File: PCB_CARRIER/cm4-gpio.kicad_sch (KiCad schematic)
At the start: 35 parts, among them J2 Micro_SD_Card_Det2, Q1 BSS138, Q2 BSS138, Q3 BSS138, Q4 BC817-40, SW1 SW_DIP_x04, U4 RT9742GGJ5

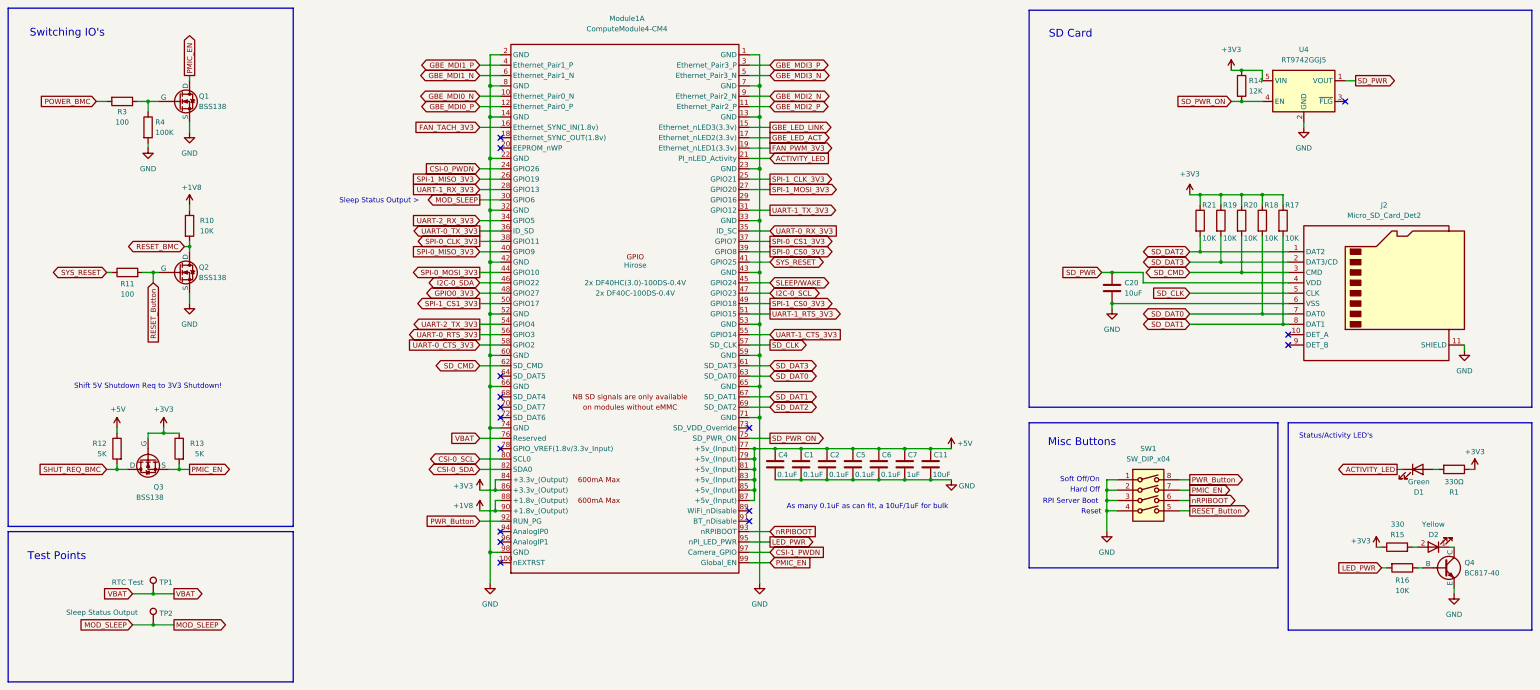
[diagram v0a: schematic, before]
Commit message: fixing another mosfet
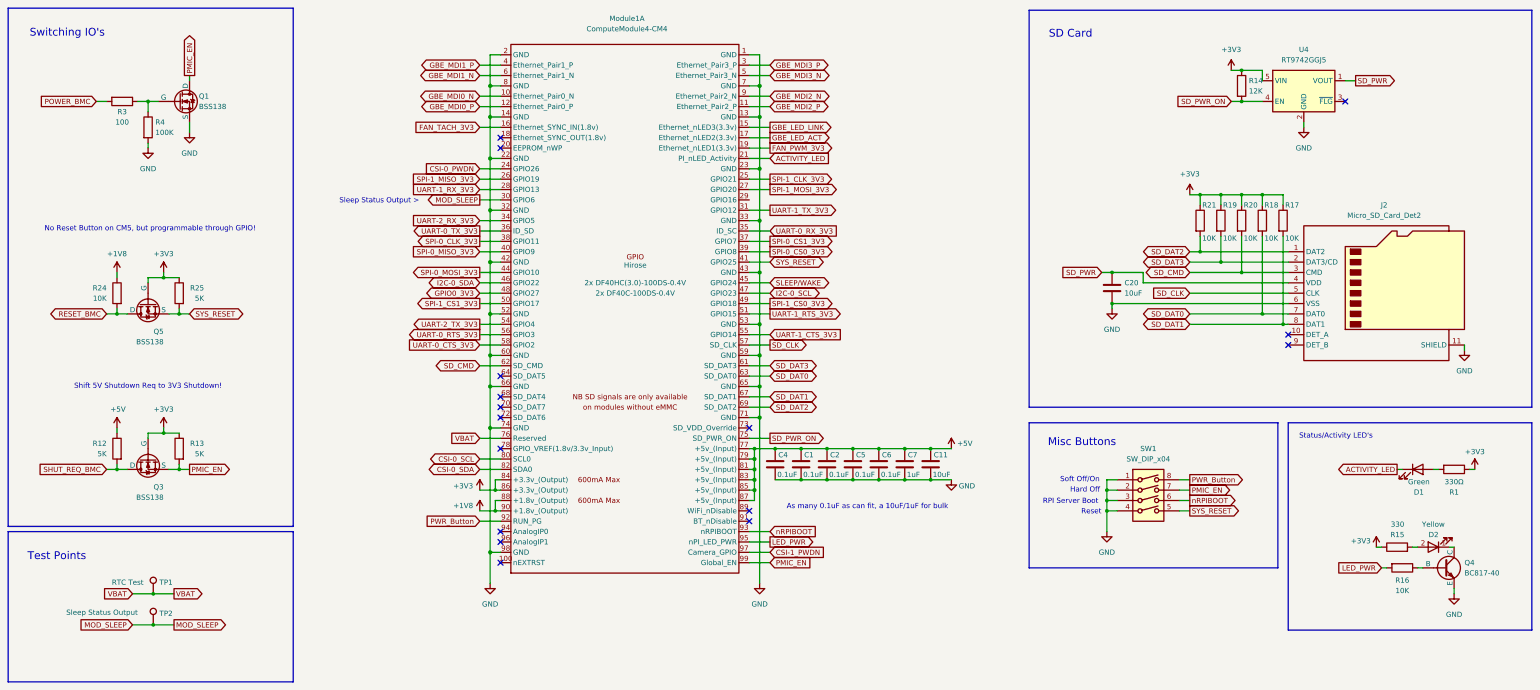
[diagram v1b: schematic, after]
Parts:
- removed Q2: BSS138, Package_TO_SOT_SMD:SOT-23-3, symbol Simulation_SPICE:NMOS
- removed R10: 10K, Resistor_SMD:R_0402_1005Metric, symbol Device:R
- removed R11: 100, Resistor_SMD:R_0402_1005Metric, symbol Device:R
- added Q5: BSS138, Package_TO_SOT_SMD:SOT-23-3, symbol Simulation_SPICE:NMOS
- added R24: 10K, Resistor_SMD:R_0402_1005Metric, symbol Device:R
- added R25: 5K, Resistor_SMD:R_0402_1005Metric, symbol Device:R
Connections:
- net RESET_Button is gone; now on net SYS_RESET: SW1.5
- net +1V8: now also R24.1
- net +3V3: now also Q5.2 (G), R25.1
- net RESET_BMC: now also Q5.1 (D), R24.2
- net SYS_RESET: now also Q5.3 (S), R25.2
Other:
- note added: "No Reset Button on CM5, but programmable through GPIO!"
